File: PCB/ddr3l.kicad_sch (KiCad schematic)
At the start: 2 parts, among them U11 MT41J128M16JT-125:K

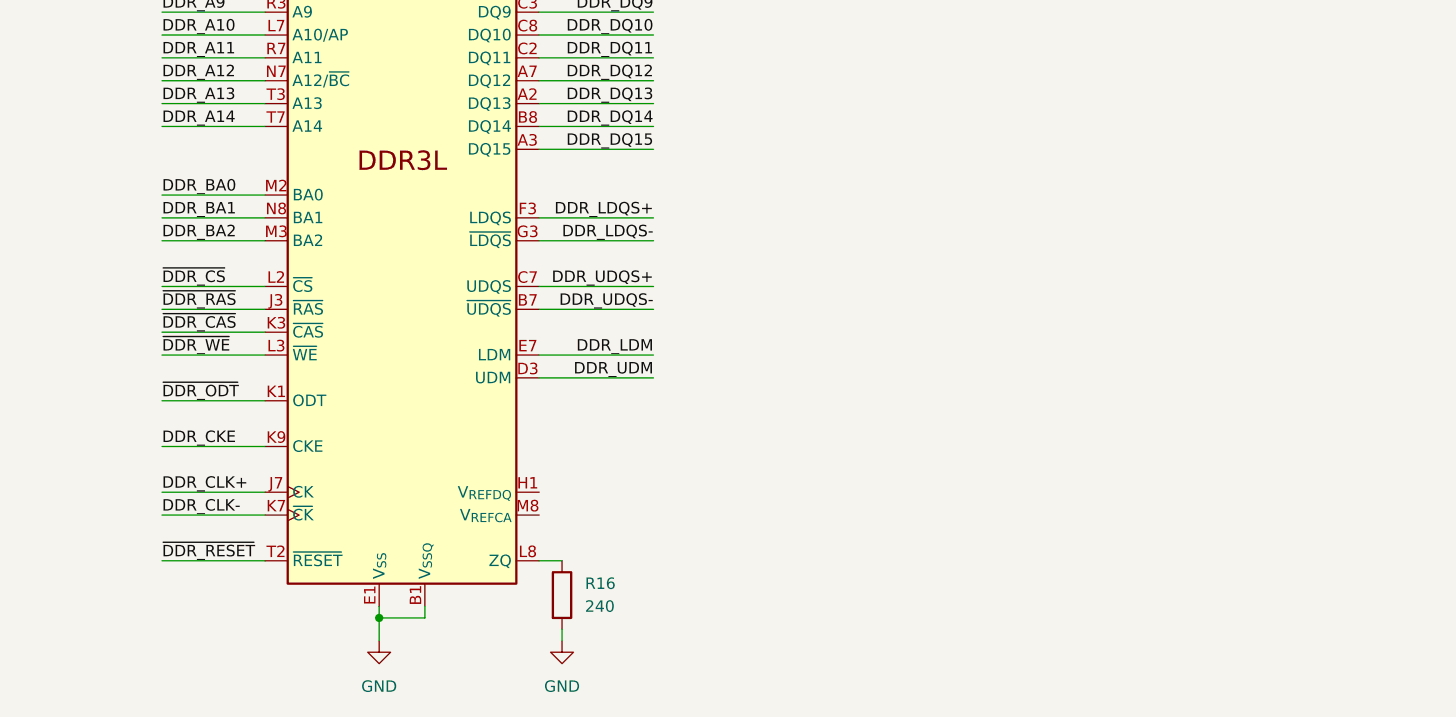
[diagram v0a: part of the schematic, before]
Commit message: VREF and other pins
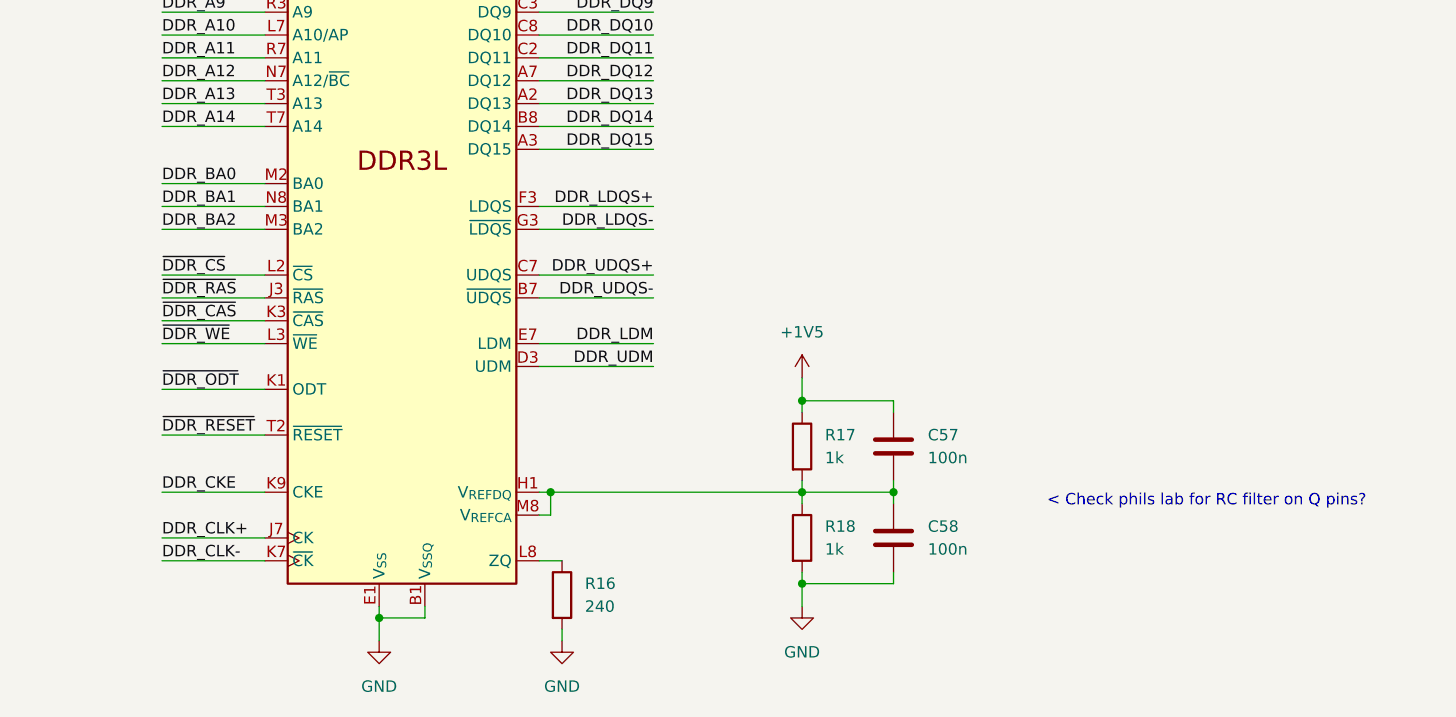
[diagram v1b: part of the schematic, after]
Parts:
- removed U11: MT41J128M16JT-125:K, Package_BGA:Micron_FBGA-96_8x14mm_Layout9x16_P0.8mm, symbol Memory_RAM:MT41K256M16TW
- added C57, C58: 100n, symbol Device:C
- added R17, R18: 1k, symbol Device:R
- added U11: MT41J128M16JT-125:K, Package_BGA:Micron_FBGA-96_8x14mm_Layout9x16_P0.8mm, symbol FPGA Accelerator:MT41J128M16JT-125{colon}K
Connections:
- net +1V5: now also C57.1, R17.1, U11.A1 (V_{DDQ}), U11.A8 (V_{DDQ}), U11.B2 (V_{DD}), U11.C1 (V_{DDQ}), U11.C9 (V_{DDQ}), U11.D2 (V_{DDQ}), U11.D9 (V_{DD}), U11.E9 (V_{DDQ}), U11.F1 (V_{DDQ}), U11.G7 (V_{DD}), U11.H2 (V_{DDQ}), U11.H9 (V_{DDQ}), U11.K2 (V_{DD}), U11.K8 (V_{DD}), U11.N1 (V_{DD}), U11.N9 (V_{DD}), U11.R1 (V_{DD}), U11.R9 (V_{DD})
- net DDR_A0: now also U11.N3 (A0)
- net DDR_A1: now also U11.P7 (A1)
- net DDR_A10: now also U11.L7 (A10/AP)
- net DDR_A11: now also U11.R7 (A11)
- net DDR_A12: now also U11.N7 (A12/~{BC})
- net DDR_A13: now also U11.T3 (A13)
- net DDR_A14: now also U11.T7 (A14)
- net DDR_A2: now also U11.P3 (A2)
- net DDR_A3: now also U11.N2 (A3)
- net DDR_A4: now also U11.P8 (A4)
- net DDR_A5: now also U11.P2 (A5)
- net DDR_A6: now also U11.R8 (A6)
- net DDR_A7: now also U11.R2 (A7)
- net DDR_A8: now also U11.T8 (A8)
- net DDR_A9: now also U11.R3 (A9)
- net DDR_BA0: now also U11.M2 (BA0)
- net DDR_BA1: now also U11.N8 (BA1)
- net DDR_BA2: now also U11.M3 (BA2)
- net DDR_CKE: now also U11.K9 (CKE)
- net DDR_CLK+: now also U11.J7 (CK)
- net DDR_CLK-: now also U11.K7 (~{CK})
- net DDR_DQ0: now also U11.E3 (DQ0)
- net DDR_DQ1: now also U11.F7 (DQ1)
- net DDR_DQ10: now also U11.C8 (DQ10)
- net DDR_DQ11: now also U11.C2 (DQ11)
- net DDR_DQ12: now also U11.A7 (DQ12)
- net DDR_DQ13: now also U11.A2 (DQ13)
- net DDR_DQ14: now also U11.B8 (DQ14)
- net DDR_DQ15: now also U11.A3 (DQ15)
- net DDR_DQ2: now also U11.F2 (DQ2)
- net DDR_DQ3: now also U11.F8 (DQ3)
- net DDR_DQ4: now also U11.H3 (DQ4)
- net DDR_DQ5: now also U11.H8 (DQ5)
- net DDR_DQ6: now also U11.G2 (DQ6)
- net DDR_DQ7: now also U11.H7 (DQ7)
- net DDR_DQ8: now also U11.D7 (DQ8)
- net DDR_DQ9: now also U11.C3 (DQ9)
- net DDR_LDM: now also U11.E7 (LDM)
- net DDR_LDQS+: now also U11.F3 (LDQS)
- net DDR_LDQS-: now also U11.G3 (~{LDQS})
- net DDR_UDM: now also U11.D3 (UDM)
- net DDR_UDQS+: now also U11.C7 (UDQS)
- net DDR_UDQS-: now also U11.B7 (~{UDQS})
- net GND: now also C58.2, R18.2, U11.A9 (V_{SS}), U11.B1 (V_{SSQ}), U11.B3 (V_{SS}), U11.B9 (V_{SSQ}), U11.D1 (V_{SSQ}), U11.D8 (V_{SSQ}), U11.E1 (V_{SS}), U11.E2 (V_{SSQ}), U11.E8 (V_{SSQ}), U11.F9 (V_{SSQ}), U11.G1 (V_{SSQ}), U11.G8 (V_{SS}), U11.G9 (V_{SSQ}), U11.J2 (V_{SS}), U11.J8 (V_{SS}), U11.M1 (V_{SS}), U11.M9 (V_{SS}), U11.P1 (V_{SS}), U11.P9 (V_{SS}), U11.T1 (V_{SS}), U11.T9 (V_{SS})
- net ~{DDR_CAS}: now also U11.K3 (~{CAS})
- net ~{DDR_CS}: now also U11.L2 (~{CS})
- net ~{DDR_ODT}: now also U11.K1 (ODT)
- net ~{DDR_RAS}: now also U11.J3 (~{RAS})
- net ~{DDR_RESET}: now also U11.T2 (~{RESET})
- net ~{DDR_WE}: now also U11.L3 (~{WE})
- net at R16.1: now also U11.L8 (ZQ)
- new net: C57.2, C58.1, R17.2, R18.1, U11.H1 (V_{REFDQ}), U11.M8 (V_{REFCA})
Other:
- note added: "< Check phils lab for RC filter on Q pins?"
